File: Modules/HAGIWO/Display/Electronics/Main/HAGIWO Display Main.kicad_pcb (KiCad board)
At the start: 2 copper layers, 27.9 x 101.6 mm, 33 parts, among them J1 Power, J2 Trigger, J3 In, J4 Out, P1 B100k, SW1 AC/DC, SW2 Encoder, U1 MCP6002-xSN

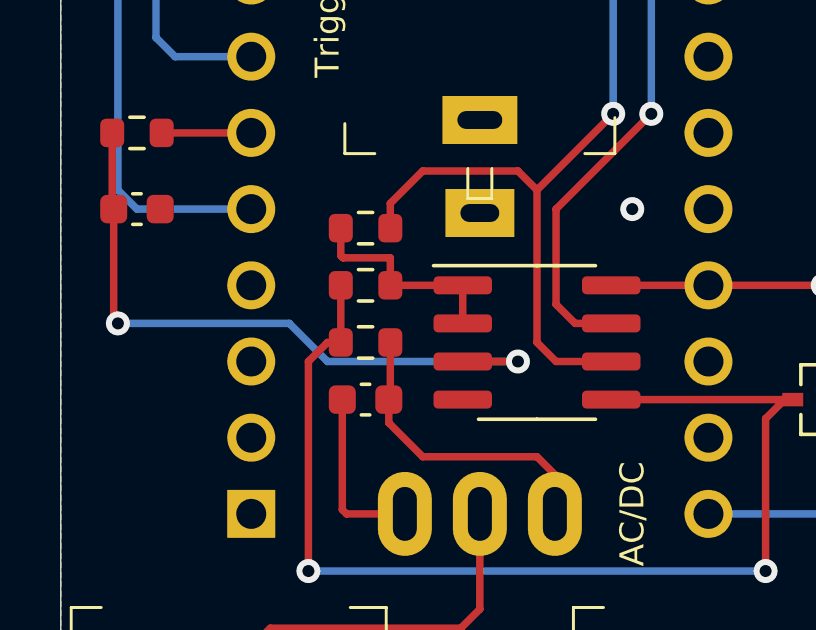
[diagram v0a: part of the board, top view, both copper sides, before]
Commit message: Bugfix
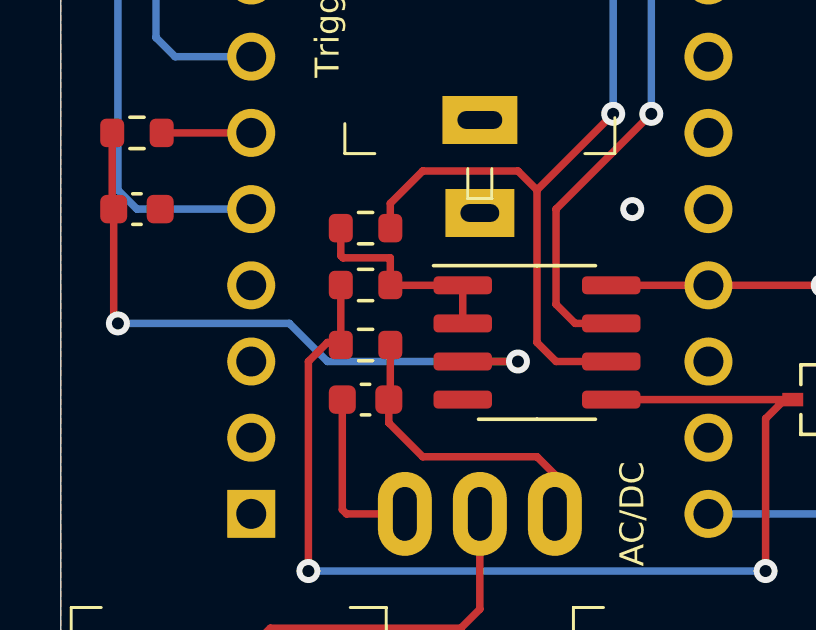
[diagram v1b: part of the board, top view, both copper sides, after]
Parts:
- moved R5 1.99 mm to (10.2, 82.0)
- moved R4 1.92 mm to (10.2, 80.0), turned to 180 degrees
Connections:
- R4 pad 1: Net-(D3-Pad3) -> Offset
- R4 pad 2: Net-(C3-Pad1) -> Net-(D3-Pad3)
- R5 pad 2: Offset -> Net-(C3-Pad1)
